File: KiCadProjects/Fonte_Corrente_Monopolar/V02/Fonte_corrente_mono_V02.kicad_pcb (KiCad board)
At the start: 2 copper layers, 90 x 100 mm, 23 parts, among them J1 Vref, J2 tensoes, J3 sinais analogicos, J4 comunicacao / sinais digitais, U1-howland1 AD828AN, U2 INA128, U3-cond1 AD828AN

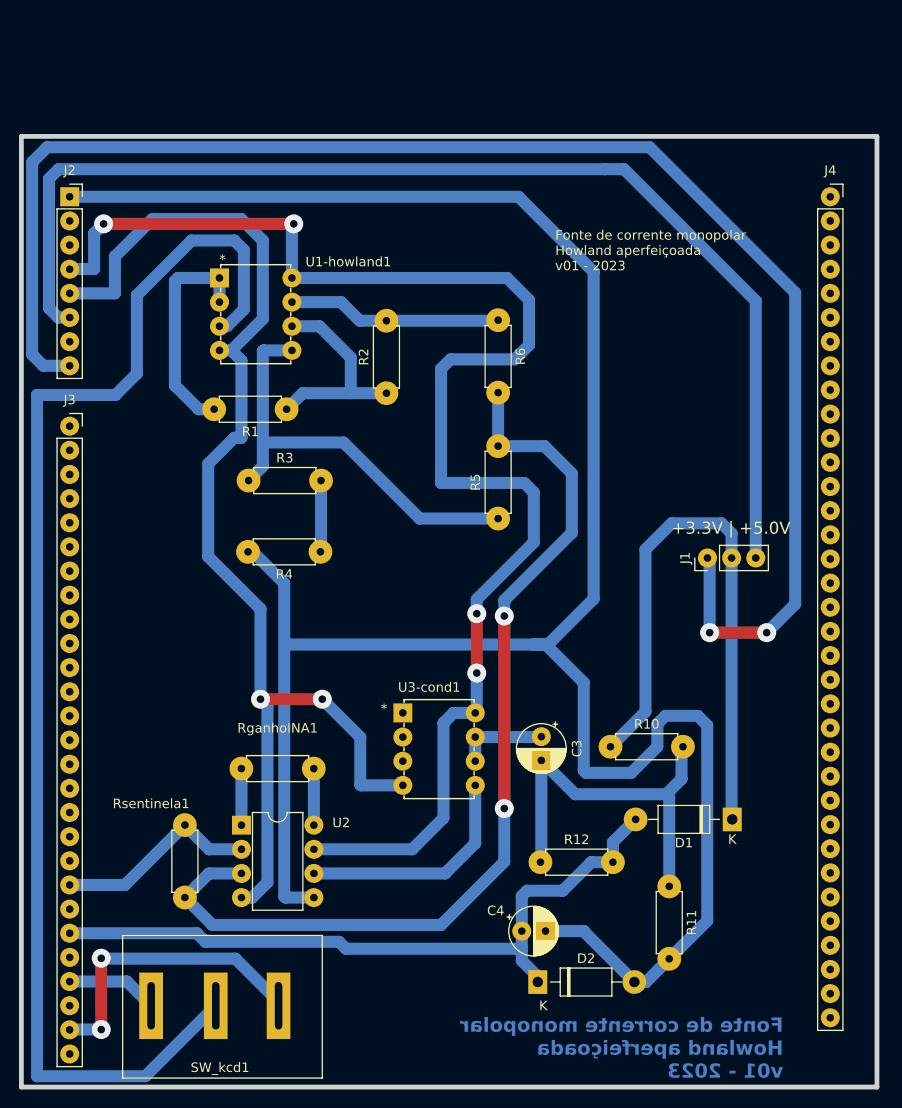
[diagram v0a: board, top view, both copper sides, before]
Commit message: baseado barramento v04
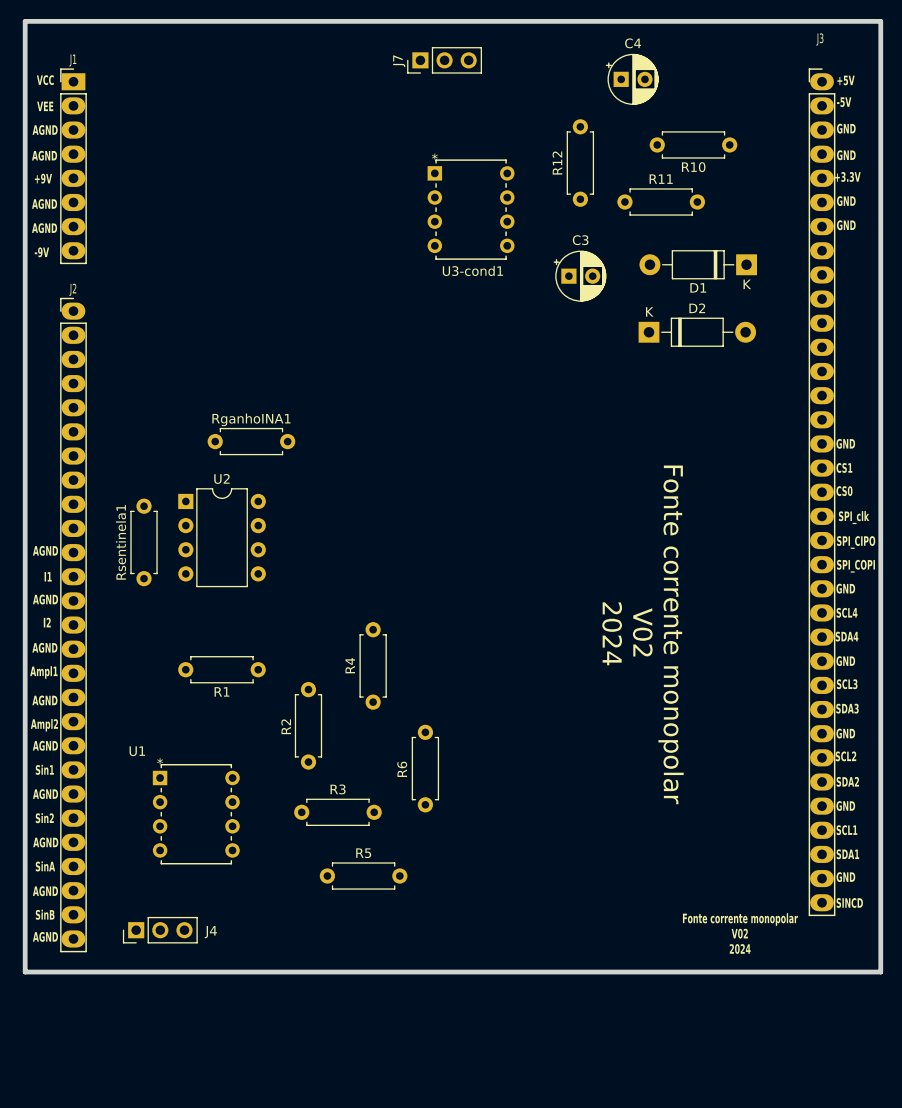
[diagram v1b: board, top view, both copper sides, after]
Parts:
- removed SW_kcd1: sw, Chave_Gangorra:chave gangorra 3 pinos
- removed U1-howland1: AD828AN, AD828AN:N_8_ADI
- added J7: Vref, Connector_PinHeader_2.54mm:PinHeader_1x03_P2.54mm_Vertical, F.Cu at (143.6, 42.8)
- added U1: AD828AN, AD828:AD828, F.Cu at (116.2, 118.3)
- J1: value Vref -> alimentacao analogica; footprint Connector_PinHeader_2.54mm:PinHeader_1x03_P2.54mm_Vertical -> Connector_PinHeader_2.54mm:PinHeader_1x08_P2.54mm_Vertical
- J2: value tensoes -> sinais analogicos; footprint Connector_PinSocket_2.54mm:PinSocket_1x08_P2.54mm_Vertical -> Connector_PinHeader_2.54mm:PinHeader_1x27_P2.54mm_Vertical
- J3: value sinais analogicos -> comunicacao / sinais digitais; footprint Connector_PinSocket_2.54mm:PinSocket_1x27_P2.54mm_Vertical -> Connector_PinHeader_2.54mm:PinHeader_1x35_P2.54mm_Vertical
- J4: value comunicacao / sinais digitais -> Change_signal; footprint Connector_PinSocket_2.54mm:PinSocket_1x35_P2.54mm_Vertical -> Connector_PinHeader_2.54mm:PinHeader_1x03_P2.54mm_Vertical
- U2: value INA128 -> INA128-H1
- U3-cond1: footprint AD828AN:N_8_ADI -> AD828:AD828
- moved J4 106.2 mm to (113.7, 134.3), turned to 90 degrees
- moved C4 90.2 mm to (164.7, 44.8)
- moved J3 87.0 mm to (185.8, 45.0)
- moved J1 83.4 mm to (107.1, 45.0), turned to 0 degrees
- moved R11 72.1 mm to (165.1, 57.7), turned to 0 degrees
- moved R12 69.9 mm to (160.4, 57.4), turned to 90 degrees
- moved D2 69.3 mm to (167.6, 71.4)
- moved R10 64.5 mm to (176.1, 51.7), turned to 180 degrees
- moved D1 58.4 mm to (177.9, 64.3)
- moved U3-cond1 56.9 mm to (145.1, 54.7)
- moved C3 48.5 mm to (159.2, 65.5), turned to 0 degrees
- moved R6 44.0 mm to (144.1, 113.5)
- moved R5 41.7 mm to (133.8, 128.6), turned to 0 degrees
- moved R3 35.3 mm to (131.1, 121.9)
- moved U2 34.5 mm to (118.9, 89.2)
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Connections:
- J1 pad 1: +3.3V -> VCC
- J1 pad 2: Net-(D1-K) -> VEE
- J1 pad 3: +5V -> Earth
- J2 pad 1: Earth -> unconnected-(J2-Pin_1-Pad1)
- J2 pad 2: VCC -> unconnected-(J2-Pin_2-Pad2)
- J2 pad 3: VEE -> unconnected-(J2-Pin_3-Pad3)
- J2 pad 4: +9V -> unconnected-(J2-Pin_4-Pad4)
- J2 pad 5: -9V -> unconnected-(J2-Pin_5-Pad5)
- J2 pad 6: +5V -> unconnected-(J2-Pin_6-Pad6)
- J2 pad 7: -5V -> unconnected-(J2-Pin_7-Pad7)
- J2 pad 8: +3.3V -> unconnected-(J2-Pin_8-Pad8)
- J3 pad 1: unconnected-(J3-Pin_1-Pad1) -> +5V
- J3 pad 16: unconnected-(J3-Pin_16-Pad16) -> Earth
- J3 pad 17: unconnected-(J3-Pin_17-Pad17) -> CS1
- J3 pad 18: unconnected-(J3-Pin_18-Pad18) -> CS0
- J3 pad 19: unconnected-(J3-Pin_19-Pad19) -> SPI_clk
- J3 pad 2: unconnected-(J3-Pin_2-Pad2) -> -5V
- J3 pad 20: I1 -> SPI_CIPO
- J3 pad 21: I2 -> SPI_COPI
- J3 pad 22: Ampl1 -> Earth
- J3 pad 23: Ampl2 -> SCL4
- J3 pad 24: Sin1 -> SDA4
- J3 pad 25: Sin2 -> Earth
- J3 pad 26: SinA -> SCL3
- J3 pad 27: SinB -> SDA3
- J3 pad 3: unconnected-(J3-Pin_3-Pad3) -> Earth
- J3 pad 4: unconnected-(J3-Pin_4-Pad4) -> Earth
- J3 pad 5: unconnected-(J3-Pin_5-Pad5) -> +3.3V
- J3 pad 6: unconnected-(J3-Pin_6-Pad6) -> Earth
- J3 pad 7: unconnected-(J3-Pin_7-Pad7) -> Earth
- J4 pad 1: SINC -> SinA
- J4 pad 2: SPI_COPI -> Net-(J4-Pin_2)
- J4 pad 3: SPI_CIPO -> Sin1
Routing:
- net Earth: track 244.0 -> 0.00 mm
- net +3.3V: track 162.9 -> 0.00 mm, vias 2 -> 0
- net +9V: track 151.1 -> 0.00 mm, vias 4 -> 0
- net Net-(U1-howland1-+IN1): track 136.8 -> 0.00 mm
- net -9V: track 126.9 -> 0.00 mm, vias 2 -> 0
- net +5V: track 123.7 -> 0.00 mm
- net out_corrente: track 102.9 -> 0.00 mm, vias 2 -> 0
- net Ampl1: track 74.5 -> 0.00 mm
- net Net-(D1-K): track 63.0 -> 0.00 mm
- net Net-(U1-howland1-+IN2): track 45.4 -> 0.00 mm
- net nó2: track 40.9 -> 0.00 mm
- net SinA: track 31.8 -> 0.00 mm, vias 2 -> 0
- net V_INA: track 24.4 -> 0.00 mm
- net out_buffer: track 23.5 -> 0.00 mm
- net Net-(U1-howland1-OUT2): track 22.5 -> 0.00 mm
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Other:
- board text added: "+3.3V"
- board text added: "+5V"
- board text added: "+9V"
- board text added: "-5V"
- board text added: "-9V"
- board text added: "AGND"
- board text added: "Ampl1"
- board text added: "Ampl2"
- board text added: "CS0"
- board text added: "CS1"
- board text added: "Fonte corrente monopolar V02 2024"
- board text added: "GND"
- board text added: "I1"
- board text added: "I2"
- board text added: "SCL1"
- board text added: "SCL2"
- board text added: "SCL3"
- board text added: "SCL4"
- board text added: "SDA1"
- board text added: "SDA2"
- board text added: "SDA3"
- board text added: "SDA4"
- board text added: "SINCD"
- board text added: "SPI_CIPO"
- board text added: "SPI_COPI"
- board text added: "SPI_clk"
- board text added: "Sin1"
- board text added: "Sin2"
- board text added: "SinA"
- board text added: "SinB"
- board text added: "VCC"
- board text added: "VEE"
- board text removed: "+3.3V | +5.0V"
- board text removed: "Fonte de corrente monopolar Howland aperfeiçoada v01 - 2023"
